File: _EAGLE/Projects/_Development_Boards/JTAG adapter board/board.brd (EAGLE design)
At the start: 40 x 60 mm, 9 parts, among them J1 PROG-HEADER_2X3_SHROUDED, J10 PROG-HEADER_2X5_1.27MM-PTH+SMD, J2 PROG-HEADER_2X5_2.00MM-SHROUD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, J3 PROG-HEADER_2X5_SHROUDED, J5 PROG-HEADER_2X10_RIGHT-ANGLE, J6 PROG-HEADER_2X10_SHROUDED, J8 CONN-1X4, J9 CONN-1X6

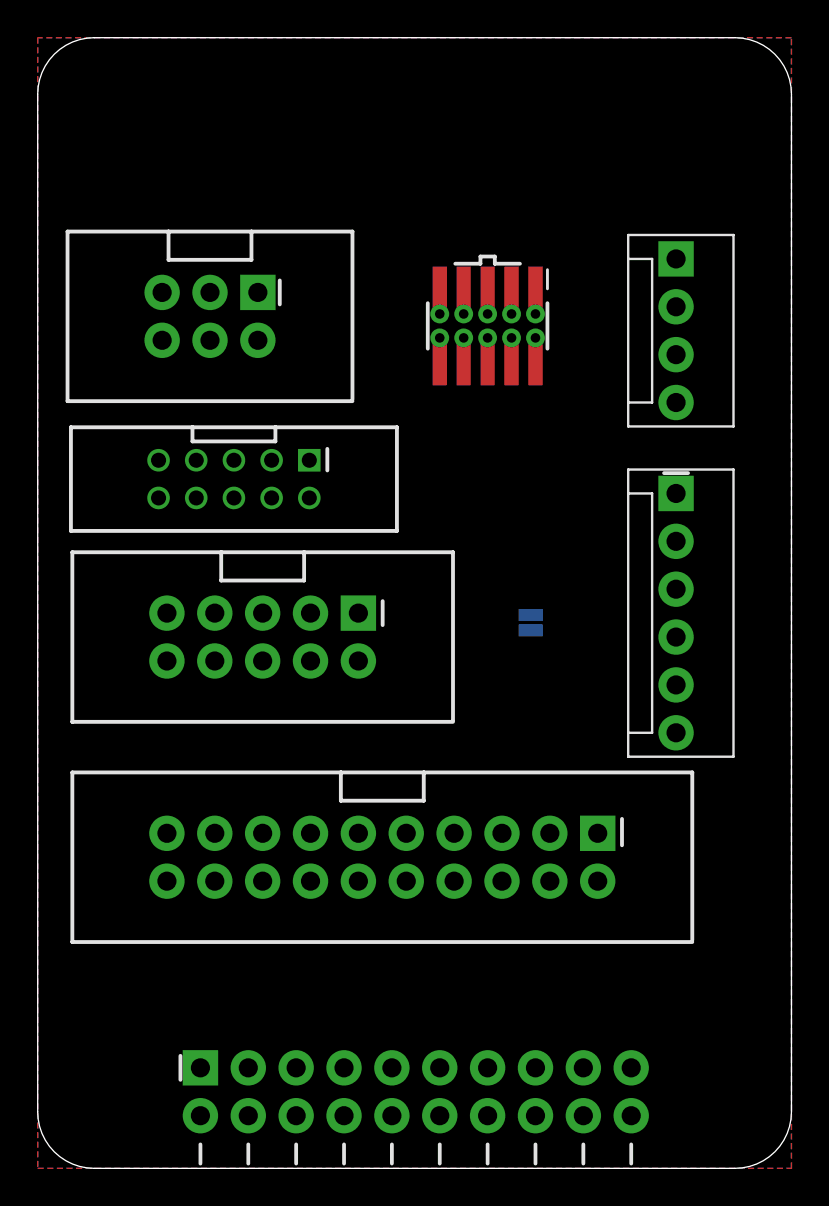
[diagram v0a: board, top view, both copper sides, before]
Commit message: JTAG board V1
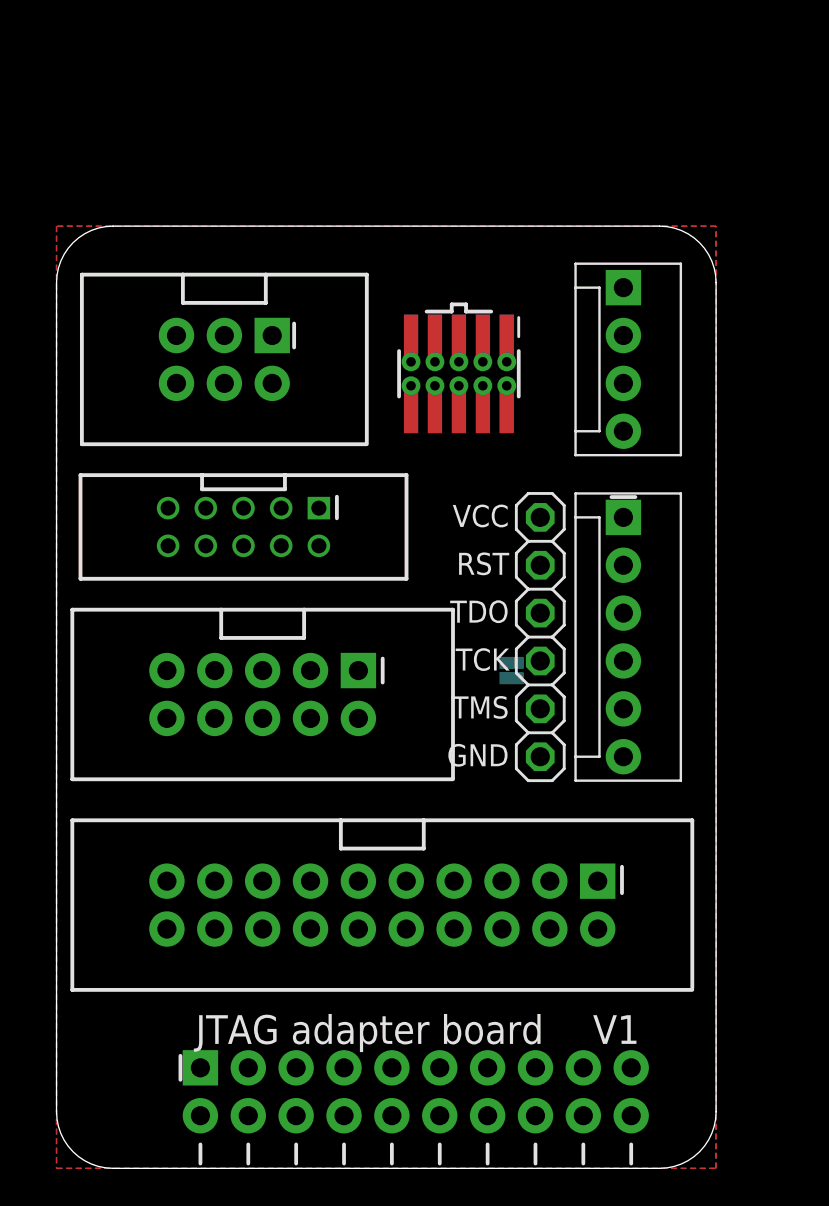
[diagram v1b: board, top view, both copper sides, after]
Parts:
- added JP2: (no value), pinhead_v2:1X06/OCT
- moved J8 3.18 mm to (31.1, 46.7)
- moved J9 3.07 mm to (31.1, 34.5)
- moved J3 3.05 mm to (11.9, 25.1)
- moved J10 2.96 mm to (22.4, 42.2)
- moved JP1 2.74 mm to (25.1, 26.4)
- moved J2 2.59 mm to (10.9, 34.0)
- moved J6 2.54 mm to (18.3, 14.0)
- moved J1 2.41 mm to (9.91, 42.9)
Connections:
- removed net N$2: J10.19, J10.9
- net GND: now also JP2.3
- net RST: now also JP2.5
- net TCK: now also JP2.2
- net TDO: now also JP2.6
- net TMS: now also JP2.4
- net VCC: now also JP2.1
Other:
- board size 40 x 60 mm -> 35 x 50 mm
- board text added: "TCK-SWCLK"
- board text added: "TDO-SWO"
- board text added: "TMS-SWDIO"
- board text removed: ">GITHUB"
- board text removed: "SWCLK"
- board text removed: "SWDIO"
- board text removed: "SWO"
- board text removed: "TCK - SWDCLK"
- board text removed: "TDO - SWO"
- board text removed: "TMS - SWDIO"
